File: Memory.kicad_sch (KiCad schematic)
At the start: 14 parts, among them IC1 NAND_MX30LF1G18AC-TI

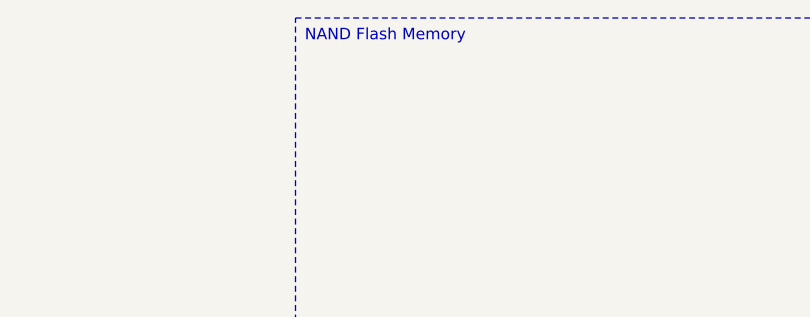
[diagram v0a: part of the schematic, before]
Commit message: Update
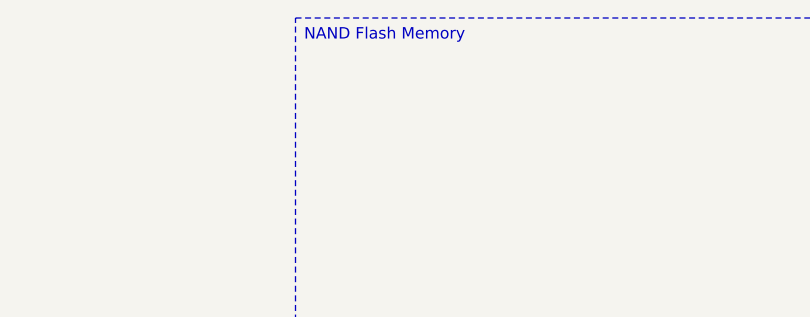
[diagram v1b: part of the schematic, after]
